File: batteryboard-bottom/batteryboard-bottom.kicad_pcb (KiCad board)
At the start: 2 copper layers, 45.6 x 45.6 mm, 34 parts, among them J1 SFC-110-T2-X-D-A, J2 FTS-107-01-X-DV-A, Q1 NX3008NBKS, Q2 MBT2222ADW1T1, Q3 NX3008NBKS, Q4 MBT2222ADW1T1, U1 INA219BxD

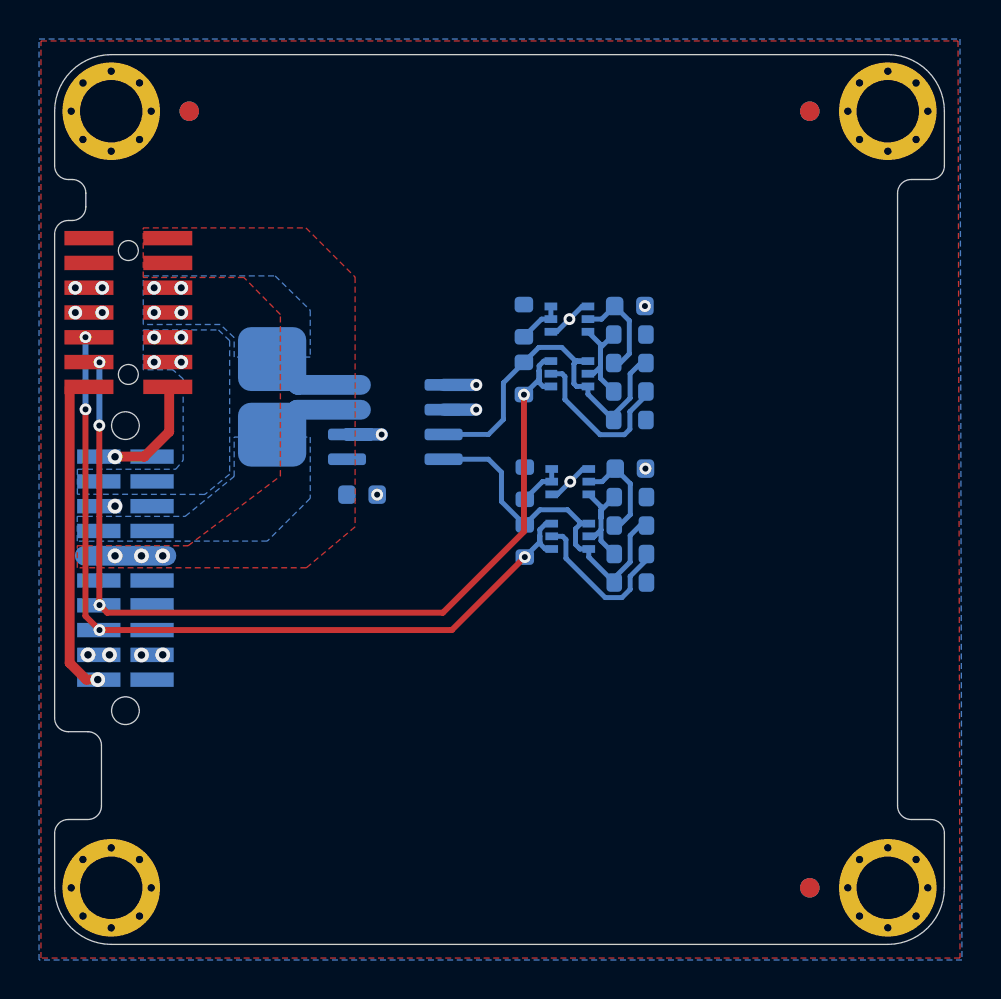
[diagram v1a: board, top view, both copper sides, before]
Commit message: Rev B3/03 updates
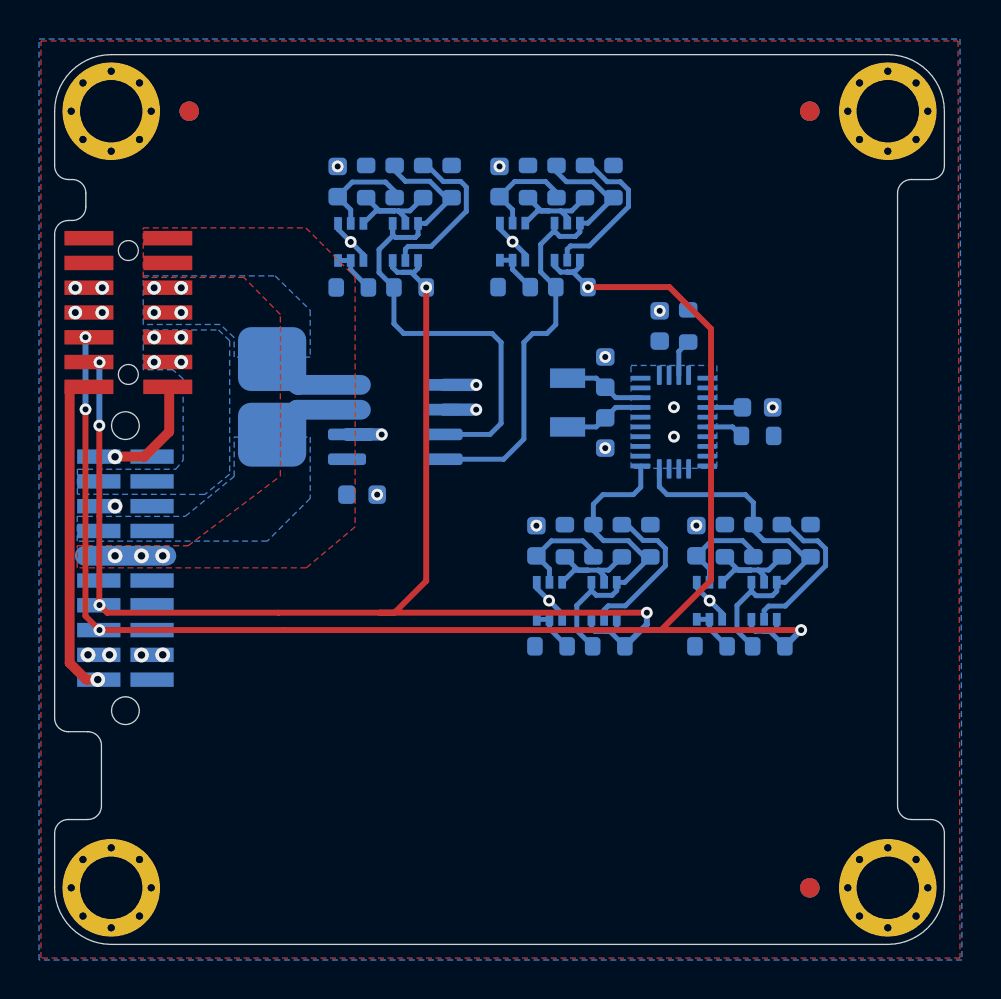
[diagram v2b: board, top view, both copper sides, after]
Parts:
- added C4: 0.1uF, Capacitor_SMD:C_0603_1608Metric, B.Cu at (112.5, 56.4)
- added C5: 0.1uF, Capacitor_SMD:C_0603_1608Metric, B.Cu at (117.5, 60.6)
- added C6: 22pF, Capacitor_SMD:C_0603_1608Metric, B.Cu at (109.7, 58.8)
- added C7: 22pF, Capacitor_SMD:C_0603_1608Metric, B.Cu at (109.7, 61.9)
- added C8: 10nF, Capacitor_SMD:C_0603_1608Metric, B.Cu at (114.4, 67.4)
- added C9: 10nF, Capacitor_SMD:C_0603_1608Metric, B.Cu at (106.2, 67.4)
- added Q5: NX3008NBKS, Package_TO_SOT_SMD:SOT-363_SC-70-6, B.Cu at (115.1, 70.5)
- added Q6: MBT2222ADW1T1, Package_TO_SOT_SMD:SOT-363_SC-70-6, B.Cu at (117.9, 70.5)
- added Q7: NX3008NBKS, Package_TO_SOT_SMD:SOT-363_SC-70-6, B.Cu at (106.9, 70.5)
- added Q8: MBT2222ADW1T1, Package_TO_SOT_SMD:SOT-363_SC-70-6, B.Cu at (109.7, 70.5)
- added R14: 680R, Resistor_SMD:R_0603_1608Metric, B.Cu at (118.8, 67.4)
- added R15: 100K, Resistor_SMD:R_0603_1608Metric, B.Cu at (115.1, 72.8)
- added R16: 10K, Resistor_SMD:R_0603_1608Metric, B.Cu at (114.0, 56.4)
- added R17: 10K, Resistor_SMD:R_0603_1608Metric, B.Cu at (117.5, 62.0)
- added R18: 10K, Resistor_SMD:R_0603_1608Metric, B.Cu at (115.8, 67.4)
- added R19: 10K, Resistor_SMD:R_0603_1608Metric, B.Cu at (120.2, 67.4)
- added R20: 200K, Resistor_SMD:R_0603_1608Metric, B.Cu at (117.3, 67.4)
- added R21: 680R, Resistor_SMD:R_0603_1608Metric, B.Cu at (110.6, 67.4)
- added R22: 100K, Resistor_SMD:R_0603_1608Metric, B.Cu at (106.9, 72.8)
- added R23: 10K, Resistor_SMD:R_0603_1608Metric, B.Cu at (107.7, 67.4)
- added R24: 10K, Resistor_SMD:R_0603_1608Metric, B.Cu at (112.0, 67.4)
- added R25: 200K, Resistor_SMD:R_0603_1608Metric, B.Cu at (109.1, 67.4)
- added R26: DNI (0R), Resistor_SMD:R_0603_1608Metric, B.Cu at (118.1, 72.8)
- added R27: DNI (0R), Resistor_SMD:R_0603_1608Metric, B.Cu at (109.9, 72.8)
- added U2: BNO085, mainboard:LGA-28, B.Cu at (113.2, 61.3)
- added Y1: 32.768kHz/12.5pF, Crystal:Crystal_SMD_MicroCrystal_CC7V-T1A-2Pin_3.2x1.5mm, B.Cu at (107.8, 60.3)
- moved R5 20.6 mm to (110.1, 49.0), turned to -90 degrees
- moved R2 19.2 mm to (108.7, 49.0), turned to -90 degrees
- moved R6 18.0 mm to (107.2, 49.0), turned to -90 degrees
- moved R4 17.0 mm to (105.8, 49.0), turned to -90 degrees
- moved C2 16.3 mm to (96.0, 49.0), turned to 90 degrees
- moved C1 16.2 mm to (104.3, 49.0), turned to 90 degrees
- moved R9 15.6 mm to (97.5, 49.0), turned to -90 degrees
- moved R10 15.3 mm to (101.8, 49.0), turned to -90 degrees
- moved R11 15.2 mm to (98.9, 49.0), turned to -90 degrees
- moved Q2 15.1 mm to (107.8, 52.1), turned to 90 degrees
- moved R7 15.1 mm to (100.4, 49.0), turned to -90 degrees
- moved R12 13.2 mm to (108.0, 54.4), turned to 0 degrees
- moved Q1 12.6 mm to (105.0, 52.1), turned to 90 degrees
- moved Q3 11.9 mm to (96.7, 52.1), turned to 90 degrees
- moved Q4 10.8 mm to (99.5, 52.1), turned to 90 degrees
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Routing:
- net SCL1: track 42.2 -> 84.1 mm, vias 4 -> 5
- net SDA1: track 46.9 -> 68.3 mm, vias 4 -> 5
- net SCL_IMU: track 0.00 -> 19.1 mm
- net SDA_IMU: track 0.00 -> 17.2 mm
- net SDA_C_SENSE: track 18.7 -> 27.0 mm
- net Net-(Q8A-B1): track 0.00 -> 8.19 mm
- net Net-(Q6A-B1): track 0.00 -> 8.18 mm
- net SCL_C_SENSE: track 18.6 -> 25.5 mm
- net Net-(Q5A-D1): track 0.00 -> 5.95 mm
- net Net-(Q7A-D1): track 0.00 -> 5.81 mm
- net Net-(Q5B-G1): track 0.00 -> 5.38 mm
- net Net-(Q7B-G1): track 0.00 -> 5.38 mm
- net GND: track 11.2 -> 16.1 mm, vias 13 -> 23
- net Net-(U2-XIN32): track 0.00 -> 4.16 mm
- net Net-(U2-CLKSEL1/XOUT32): track 0.00 -> 4.16 mm
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- added copper zone on B.Cu, net GND
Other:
- board text added: "30-JAN-23"
- board text added: "Rev B3/03"
- board text removed: "12-APR-23"
- board text removed: "Rev B3/02"
